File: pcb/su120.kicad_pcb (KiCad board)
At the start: 2 copper layers, 98.8 x 98 mm, 298 parts, among them J1 MJ-4PP-9, J2 Conn_01x03, J3 Conn_01x08, J4 Conn_01x08, J5 Conn_01x03, J6 MJ-4PP-9, SW1 SW_Push, SW10 SW_Push, SW11 SW_Push, SW12 SW_Push, SW13 SW_Push, SW14 SW_Push, SW15 SW_Push, SW16 SW_Push, SW17 SW_Push, SW18 SW_Push, SW19 SW_Push, SW2 SW_Push, SW20 SW_Push, SW21 SW_Push, SW3 SW_Push, SW4 SW_Push, SW5 SW_Push, SW6 SW_Push, SW7 SW_Push, SW8 SW_Push, SW9 SW_Push, U1 ProMicro

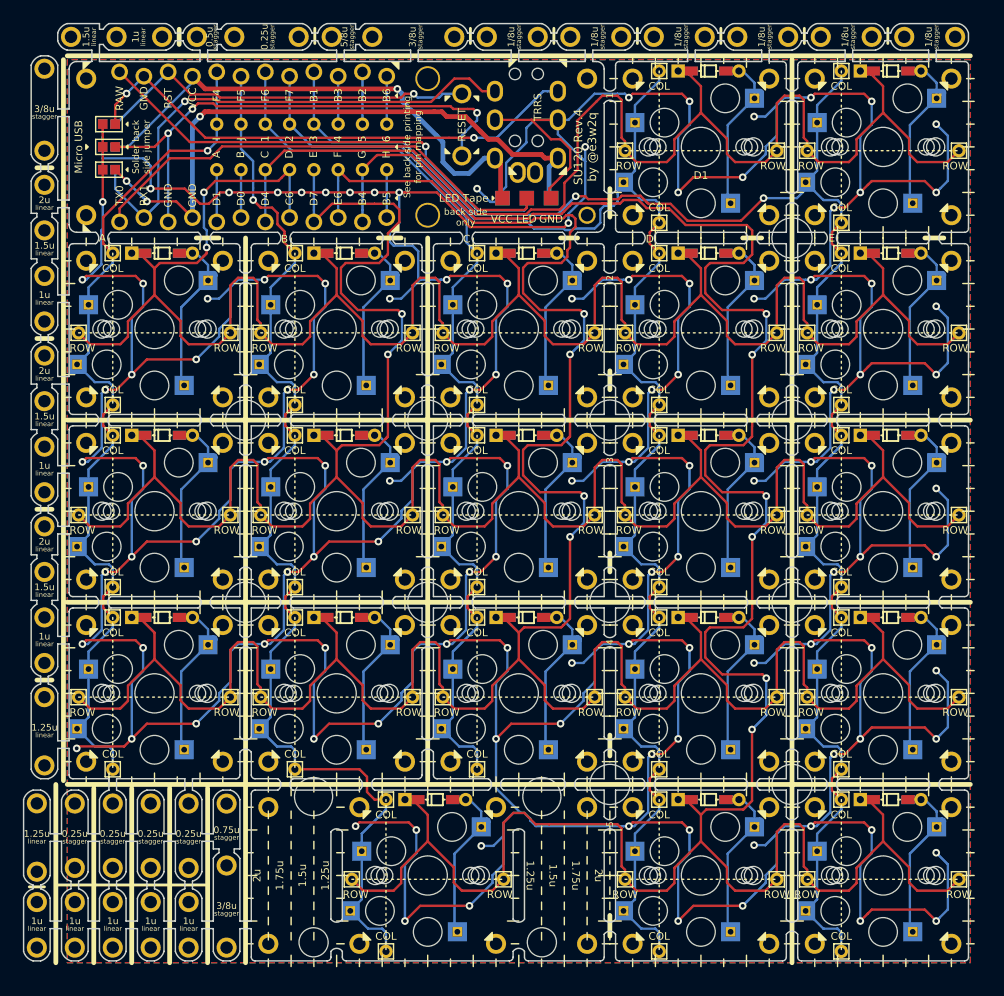
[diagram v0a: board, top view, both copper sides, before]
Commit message: rev5
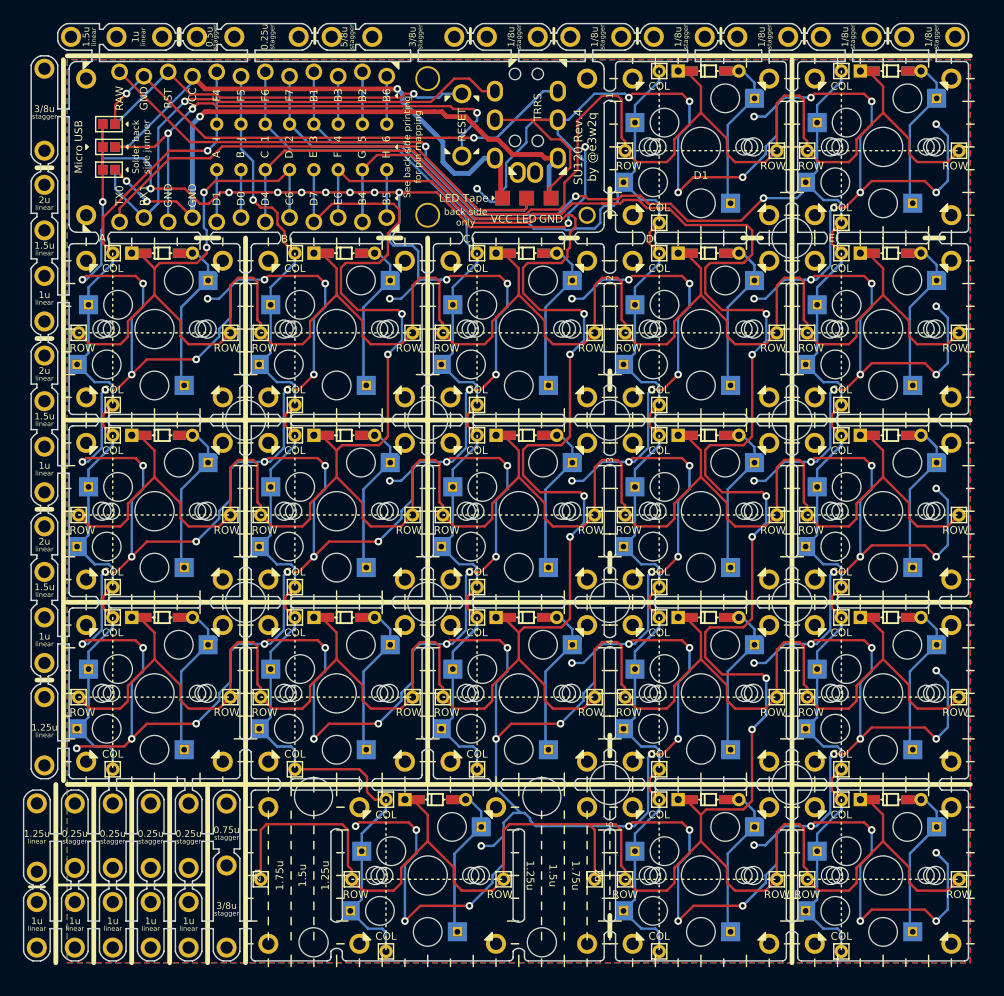
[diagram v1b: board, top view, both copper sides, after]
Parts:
- added H49: MountingHole_Pad, #footprint:1pin_conn, F.Cu at (62.7, 143.3)
- added H50: MountingHole_Pad, #footprint:1pin_conn, F.Cu at (97.6, 143.3)
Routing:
- net Y5: track 278.0 -> 302.6 mm
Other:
- outline, holes or cut-outs redrawn

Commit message: Rev6
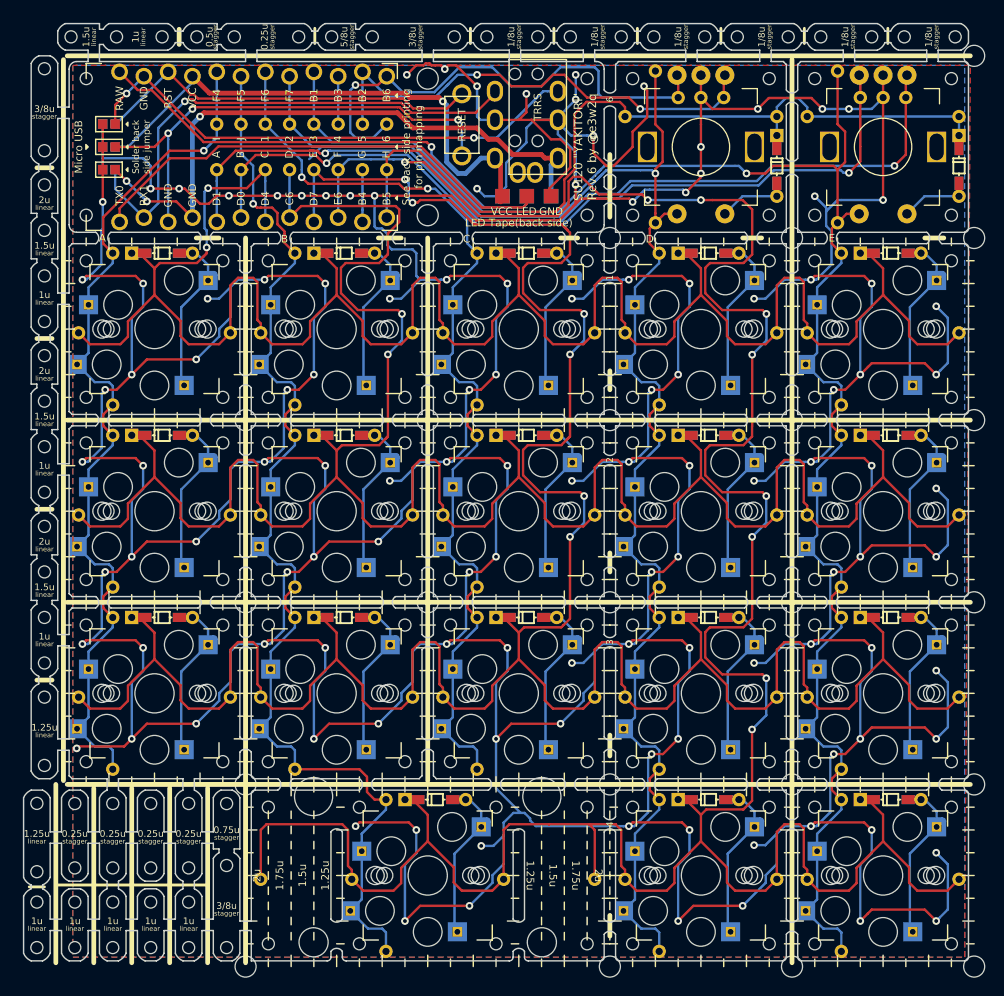
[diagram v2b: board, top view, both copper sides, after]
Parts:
- added ?: , #footprint:CherryMX_MidHeight_Choc_Silk_Line, F.Cu at (90.5, 143.3)
- added ?: , #footprint:CherryMX_MidHeight_Choc_Silk, F.Cu at (127.8, 142.9)
- added ?: , #footprint:CherryMX_MidHeight_Choc_Silk, F.Cu at (108.7, 142.9)
- added ?: , #footprint:CherryMX_MidHeight_Choc_Silk, F.Cu at (80.2, 142.9)
- added ?: , #footprint:CherryMX_MidHeight_Choc_Silk, F.Cu at (51.6, 123.8)
- added ?: , #footprint:CherryMX_MidHeight_Choc_Silk, F.Cu at (70.6, 123.8)
- added ?: , #footprint:CherryMX_MidHeight_Choc_Silk, F.Cu at (89.7, 123.8)
- added ?: , #footprint:CherryMX_MidHeight_Choc_Silk, F.Cu at (108.7, 123.8)
- added ?: , #footprint:CherryMX_MidHeight_Choc_Silk, F.Cu at (127.8, 123.8)
- added ?: , #footprint:CherryMX_MidHeight_Choc_Silk, F.Cu at (127.8, 104.8)
- added ?: , #footprint:CherryMX_MidHeight_Choc_Silk, F.Cu at (108.7, 104.8)
- added ?: , #footprint:CherryMX_MidHeight_Choc_Silk, F.Cu at (89.7, 104.8)
- added ?: , #footprint:CherryMX_MidHeight_Choc_Silk, F.Cu at (70.6, 104.8)
- added ?: , #footprint:CherryMX_MidHeight_Choc_Silk, F.Cu at (51.6, 104.8)
- added ?: , #footprint:CherryMX_MidHeight_Choc_Silk, F.Cu at (51.6, 85.7)
- added ?: , #footprint:CherryMX_MidHeight_Choc_Silk, F.Cu at (70.6, 85.7)
- added ?: , #footprint:CherryMX_MidHeight_Choc_Silk, F.Cu at (89.7, 85.7)
- added ?: , #footprint:CherryMX_MidHeight_Choc_Silk, F.Cu at (127.8, 85.7)
- added ?: , #footprint:CherryMX_MidHeight_Choc_Silk, F.Cu at (108.7, 85.7)
- added ?: , #footprint:CherryMX_MidHeight_Choc_Silk_Line, F.Cu at (70.2, 143.3)
- added ?: , #footprint:CherryMX_MidHeight_Choc_Silk_Line, F.Cu at (123.0, 66.7)
- added ?: , #footprint:CherryMX_MidHeight_Choc_Silk_Line, F.Cu at (104.0, 66.7)
- added ?: , #footprint:CherryMX_MidHeight_Choc_Silk_Line, F.Cu at (108.7, 63.5)
- added ?: , #footprint:CherryMX_MidHeight_Choc_Silk_Line, F.Cu at (127.8, 63.5)
- added ?: , #footprint:M2_Hole, F.Cu at (61.1, 152.4)
- added ?: , #footprint:M2_Hole, F.Cu at (137.3, 57.2)
- added ?: , #footprint:M2_Hole, F.Cu at (61.1, 133.3)
- added ?: , #footprint:M2_Hole, F.Cu at (99.2, 152.4)
- added ?: , #footprint:M2_Hole, F.Cu at (118.3, 152.4)
- added ?: , #footprint:M2_Hole, F.Cu at (137.3, 152.4)
- added ?: , #footprint:M2_Hole, F.Cu at (137.3, 133.3)
- added ?: , #footprint:M2_Hole, F.Cu at (137.3, 114.3)
- added ?: , #footprint:M2_Hole, F.Cu at (137.3, 95.2)
- added ?: , #footprint:M2_Hole, F.Cu at (137.3, 76.2)
- added ?: , #footprint:M2_Hole, F.Cu at (99.2, 76.2)
- added H51: MountingHole_Pad, #footprint:1pin_conn, F.Cu at (111.1, 61.5)
- added H52: MountingHole_Pad, #footprint:1pin_conn, F.Cu at (127.8, 61.5)
- added H53: MountingHole_Pad, #footprint:1pin_conn, F.Cu at (106.4, 61.5)
- added H54: MountingHole_Pad, #footprint:1pin_conn, F.Cu at (130.2, 61.5)
- added H55: MountingHole_Pad, #footprint:1pin_conn, F.Cu at (108.7, 61.5)
- added H56: MountingHole_Pad, #footprint:1pin_conn, F.Cu at (125.4, 61.5)
- ? (x147): footprint #footprint:M1.4_tapping_Pad -> #footprint:M1.4_tapping_Hole
- ? (x11): footprint #footprint:M2_spacer -> #footprint:M2_Hole
- ? (x2): footprint #footprint:M2 -> #footprint:M2_Hole
- ?: footprint #footprint:M1.4_tapping_Pad_1.8mm -> #footprint:M1.4_tapping_Hole
- SW1, SW10, SW11, SW12, SW13, SW14, SW15, SW16, SW17, SW2, SW21, SW3, SW4, SW5, SW6, SW7, SW8, SW9: footprint #footprint:CherryMX_Choc_Hotswap_rev4 -> #footprint:CherryMX_MidHeight_Choc_Hotswap_rev5
- SW19, SW20: value SW_Push -> Rotary_Encoder_Switch; footprint #footprint:CherryMX_Choc_Hotswap_rev4 -> #footprint:RotaryEncoder_Alps_EC11E-Switch_Vertical_H20mm_rev2
- U1: footprint #footprint:ArduinoProMicro-ZigZag_rev4 -> #footprint:ArduinoProMicro-ZigZag_rev5
- moved D18 12.2 mm to (116.7, 65.9), turned to 270 degrees
- moved D19 12.2 mm to (135.7, 65.9), turned to 270 degrees
- moved H137 3.57 mm to (100.8, 63.5)
- moved H138 3.57 mm to (116.7, 63.5)
- moved H139 3.57 mm to (119.9, 63.5)
- moved H140 3.57 mm to (135.7, 63.5)
- moved H136 0.40 mm to (123.0, 74.6)
- moved H135 0.40 mm to (104.0, 74.6)
- moved H133 0.40 mm to (104.0, 58.7)
- moved H134 0.40 mm to (123.0, 58.7)
- moved J2 0.20 mm to (88.0, 71.8)
- moved J5 0.20 mm to (93.1, 71.8)
- turned SW19 to 270 degrees
- turned SW20 to 270 degrees
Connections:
- D1 pad 1: Y2 -> Y1
- D10 pad 1: Y3 -> Y2
- D11 pad 1: Y4 -> Y3
- D12 pad 1: Y4 -> Y3
- D13 pad 1: Y4 -> Y3
- D14 pad 1: Y4 -> Y3
- D15 pad 1: Y4 -> Y3
- D16 pad 1: Y5 -> Y4
- D17 pad 1: Y5 -> Y4
- D18 pad 1: Y1 -> Y6
- D19 pad 1: Y1 -> Y6
- D2 pad 1: Y2 -> Y1
- D20 pad 1: Y5 -> Y4
- D3 pad 1: Y2 -> Y1
- D4 pad 1: Y2 -> Y1
- D5 pad 1: Y2 -> Y1
- D6 pad 1: Y3 -> Y2
- D7 pad 1: Y3 -> Y2
- D8 pad 1: Y3 -> Y2
- D9 pad 1: Y3 -> Y2
- H11 pad 1: Y2 -> Y1
- H12 pad 1: Y2 -> Y1
- H123 pad 1: Y4 -> Y3
- H124 pad 1: Y4 -> Y3
- H125 pad 1: Y4 -> Y3
- H126 pad 1: Y4 -> Y3
- H127 pad 1: Y4 -> Y3
- H128 pad 1: Y4 -> Y3
- H129 pad 1: Y4 -> Y3
- H13 pad 1: Y2 -> Y1
- H130 pad 1: Y4 -> Y3
- H131 pad 1: Y4 -> Y3
- H132 pad 1: Y4 -> Y3
- H137 pad 1: Y1 -> Y6
- H138 pad 1: Y1 -> Y6
- H139 pad 1: Y1 -> Y6
- H14 pad 1: Y2 -> Y1
- H140 pad 1: Y1 -> Y6
- H15 pad 1: Y2 -> Y1
- H16 pad 1: Y2 -> Y1
- H17 pad 1: Y2 -> Y1
- H18 pad 1: Y2 -> Y1
- H19 pad 1: Y2 -> Y1
- H20 pad 1: Y2 -> Y1
- H212 pad 1: Y5 -> Y4
- H213 pad 1: Y5 -> Y4
- H31 pad 1: Y3 -> Y2
- H32 pad 1: Y3 -> Y2
- H33 pad 1: Y3 -> Y2
- H34 pad 1: Y3 -> Y2
- H35 pad 1: Y3 -> Y2
- H36 pad 1: Y3 -> Y2
- H37 pad 1: Y3 -> Y2
- H38 pad 1: Y3 -> Y2
- H39 pad 1: Y3 -> Y2
- H40 pad 1: Y3 -> Y2
- H45 pad 1: Y5 -> Y4
- H46 pad 1: Y5 -> Y4
- H47 pad 1: Y5 -> Y4
- H48 pad 1: Y5 -> Y4
- H49 pad 1: Y5 -> Y4
- H50 pad 1: Y5 -> Y4
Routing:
- net Y5: track 302.6 -> 5.47 mm, vias 6 -> 0
- net Y1: track 136.7 -> 234.4 mm, vias 0 -> 2
- net X9: track 5.47 -> 95.4 mm, vias 0 -> 2
- net Y6: track 5.01 -> 92.0 mm
- net X10: track 5.04 -> 86.9 mm, vias 0 -> 2
- net X8: track 5.01 -> 52.5 mm, vias 0 -> 1
- net Y3: track 264.7 -> 312.1 mm, vias 2 -> 6
- net X7: track 5.47 -> 50.9 mm, vias 0 -> 2
- net Y2: track 236.5 -> 266.4 mm
- net X4: track 163.1 -> 184.3 mm, vias 0 -> 1
- net GND: track 988.5 -> 1009.4 mm, vias 117 -> 122
- net Net-(D18-Pad2): track 18.2 -> 8.90 mm
- net Net-(D19-Pad2): track 18.2 -> 8.90 mm
- net reset1: track 55.2 -> 52.1 mm
- net dummyVCC: track 55.7 -> 57.8 mm
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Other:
- outline, holes or cut-outs redrawn
- board text added: "LED Tape(back side)"
- board text added: "SU120 "YAKITORI" Rev.6 by @e3w2q"
- board text removed: "LED Tape"
- board text removed: "SU120 Rev.4 by @e3w2q"
- board text removed: "back side only"
